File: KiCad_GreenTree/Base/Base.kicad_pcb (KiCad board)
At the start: 2 copper layers, 65 x 62.2 mm, 46 parts, among them Q1 BCX56, Q2 BCX56, Q3 BCX56, Q4 BCX56, SW1 SW_DPDT_x2, U1 NE555D, U2 NE555D, U3 74HC04, U4 L78L05_TO92

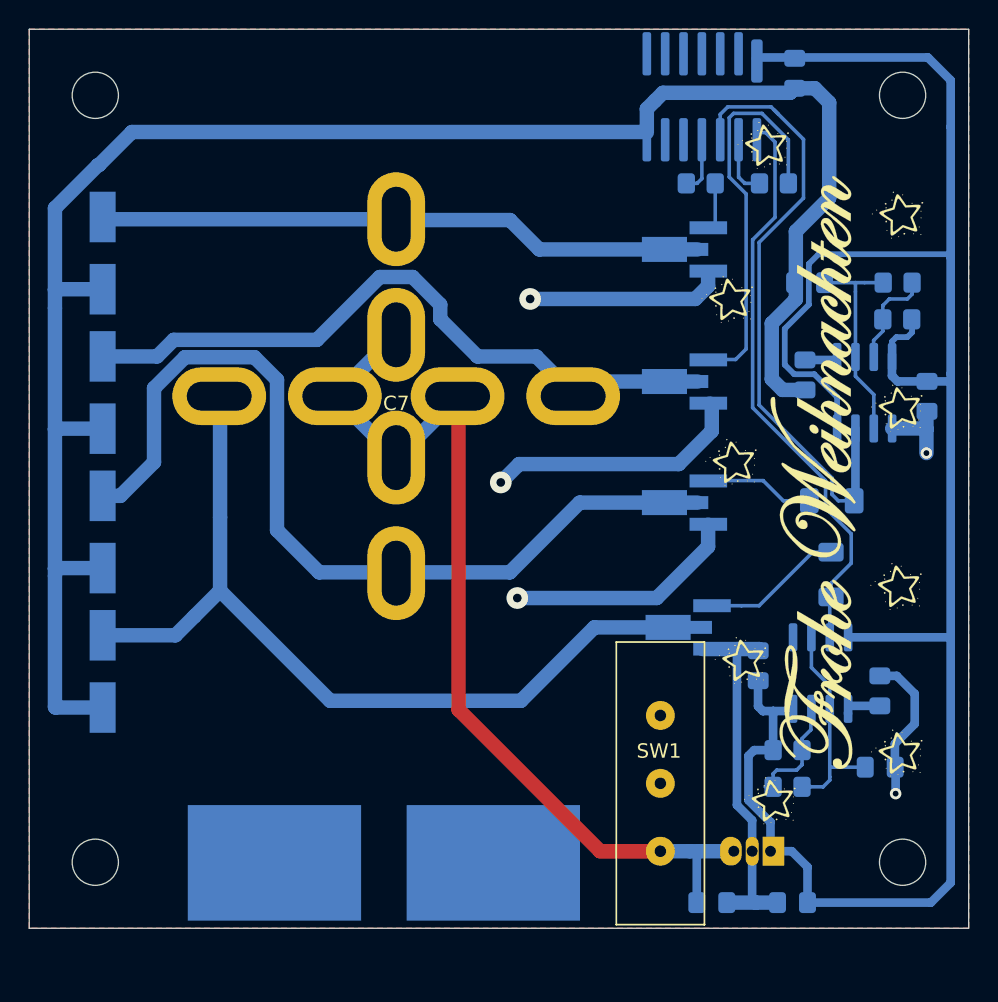
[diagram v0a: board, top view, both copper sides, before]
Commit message: Base V2.0
Finished Rework. Sould now work. Hoping for the best
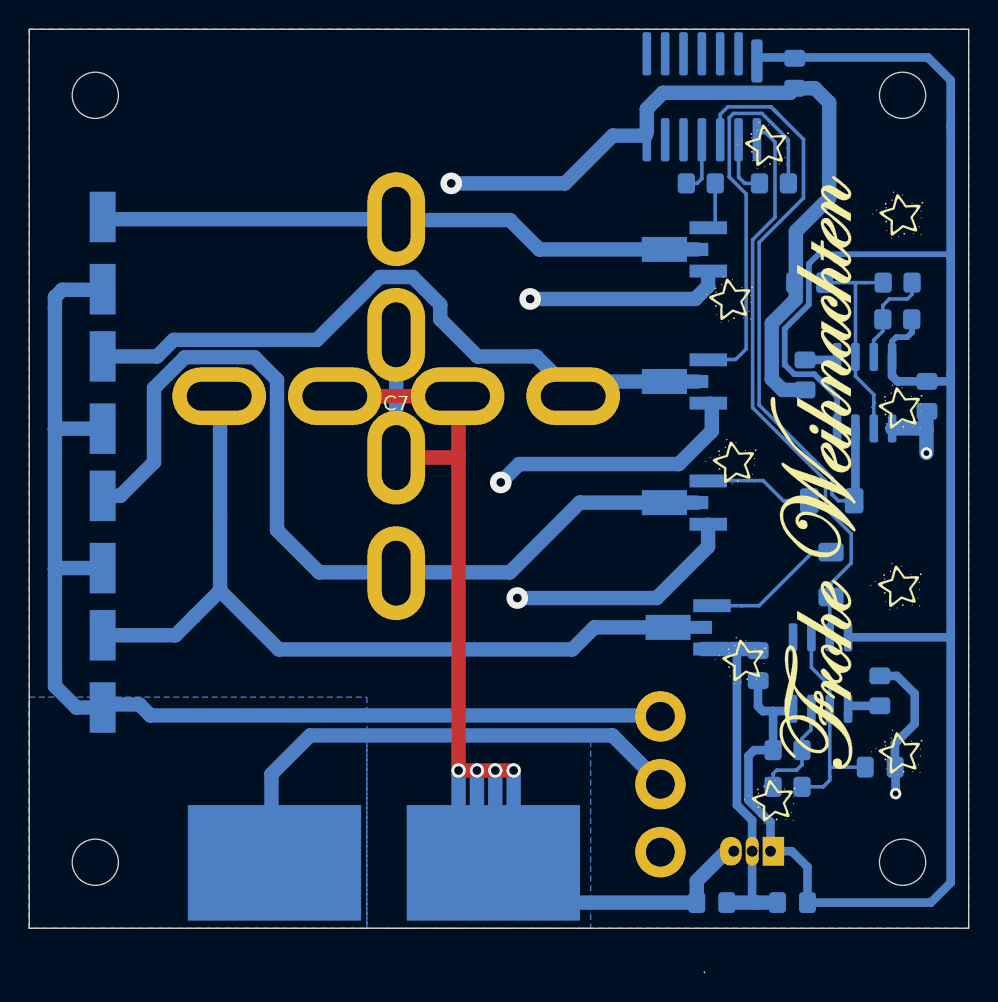
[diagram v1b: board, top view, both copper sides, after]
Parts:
- moved SW1 3.30 mm to (158.5, 112.7)
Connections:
- BT3 pad 1: Net-(BT3-Pad1) -> VCC
- BT3 pad 2: GND -> Net-(BT3-Pad2)
- D1 pad 1: GND -> GND2
- D2 pad 1: GND -> GND2
- D3 pad 1: GND -> GND2
- D4 pad 1: GND -> GND2
- SW1 pad 1: VCC -> GND
- SW1 pad 2: Net-(BT3-Pad1) -> Net-(BT3-Pad2)
- SW1 pad 3: +9V -> GND2
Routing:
- net GND2: track 0.00 -> 80.3 mm
- net GND: track 222.7 -> 142.7 mm, vias 5 -> 6
- net Net-(BT3-Pad2): track 0.00 -> 40.3 mm
- net VCC: track 66.7 -> 91.7 mm, vias 0 -> 4
- net /LED_MATRIX_1: track 59.9 -> 57.0 mm
- added copper zone on B.Cu, net Net-(BT3-Pad2)
- added copper zone on B.Cu, net VCC
